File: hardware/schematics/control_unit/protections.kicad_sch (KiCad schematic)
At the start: 6 parts, among them U17 LM35-D, U18 LM324

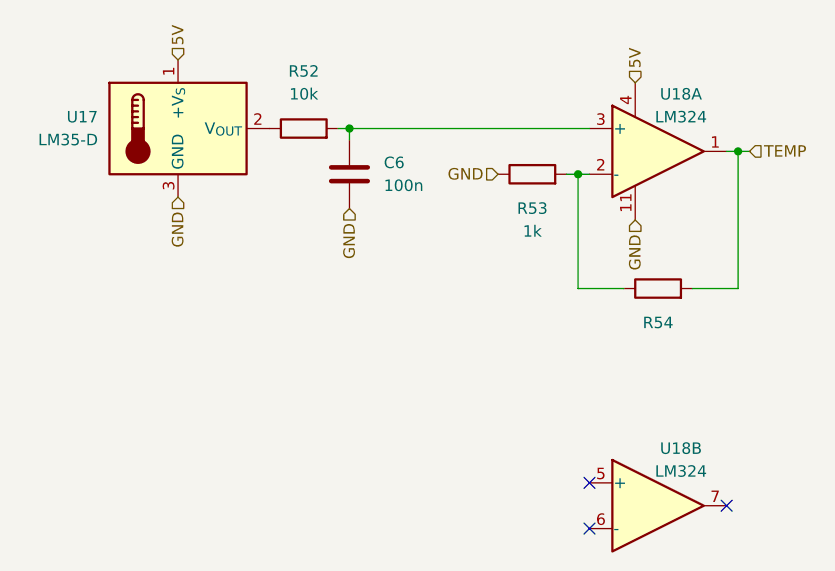
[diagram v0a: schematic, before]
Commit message: !feat
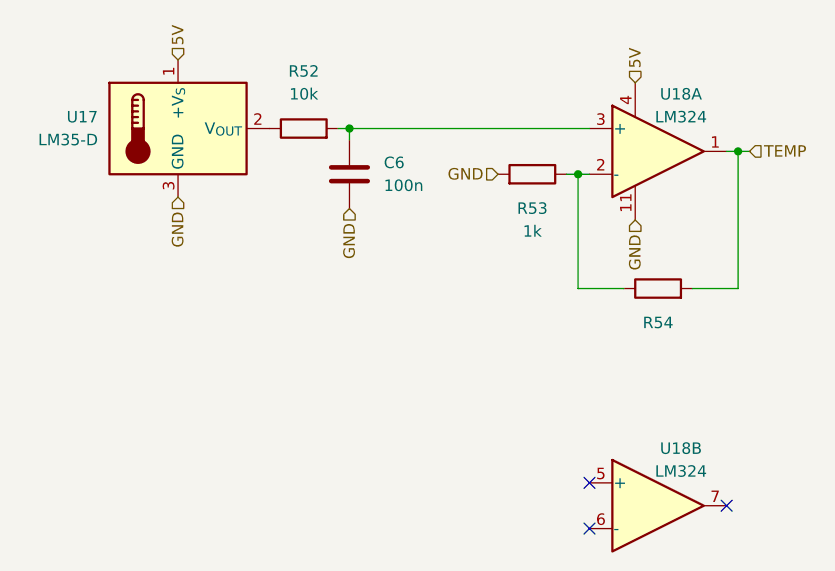
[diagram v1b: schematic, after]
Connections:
- net GND: now also R53.2; no longer R53.1
- net at R54.1, U18.2 (-): now also R53.1; no longer R53.2
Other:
- moved on the sheet: R53
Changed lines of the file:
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@@
 	(symbol
 		(lib_id "Device:R")
-		(at 151.13 80.01 90)
+		(at 151.13 80.01 270)
+		(mirror x)
 		(unit 1)
 		(exclude_from_sim no)
